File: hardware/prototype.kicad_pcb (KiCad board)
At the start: 2 copper layers, 200 x 200 mm, 111 parts, among them J1 CONN_02X20, SW1 SW_Push, SW10 SW_Push, SW11 SW_Push, SW12 SW_Push, SW13 SW_Push, SW14 SW_Push, SW15 SW_Push, SW16 SW_Push, SW17 SW_Push, SW18 SW_Push, SW19 SW_Push, SW2 SW_Push, SW20 SW_Push, SW21 SW_Push, SW22 SW_Push, SW23 SW_Push, SW24 SW_Push, SW25 SW_Push, SW26 SW_Push, SW3 SW_Push, SW4 SW_Push, SW5 SW_Push, SW6 SW_Push, SW7 SW_Push, SW8 SW_Push, SW9 SW_Push, U1 TLC5916, U10 SN74HC165N, U11 TLC5916, U2 TLC5916, U3 TLC5916, U4 SN74HC165N, U5 SN74HC165N, U6 TLC5916, U7 TLC5916, U8 TLC5916, U9 SN74HC165N

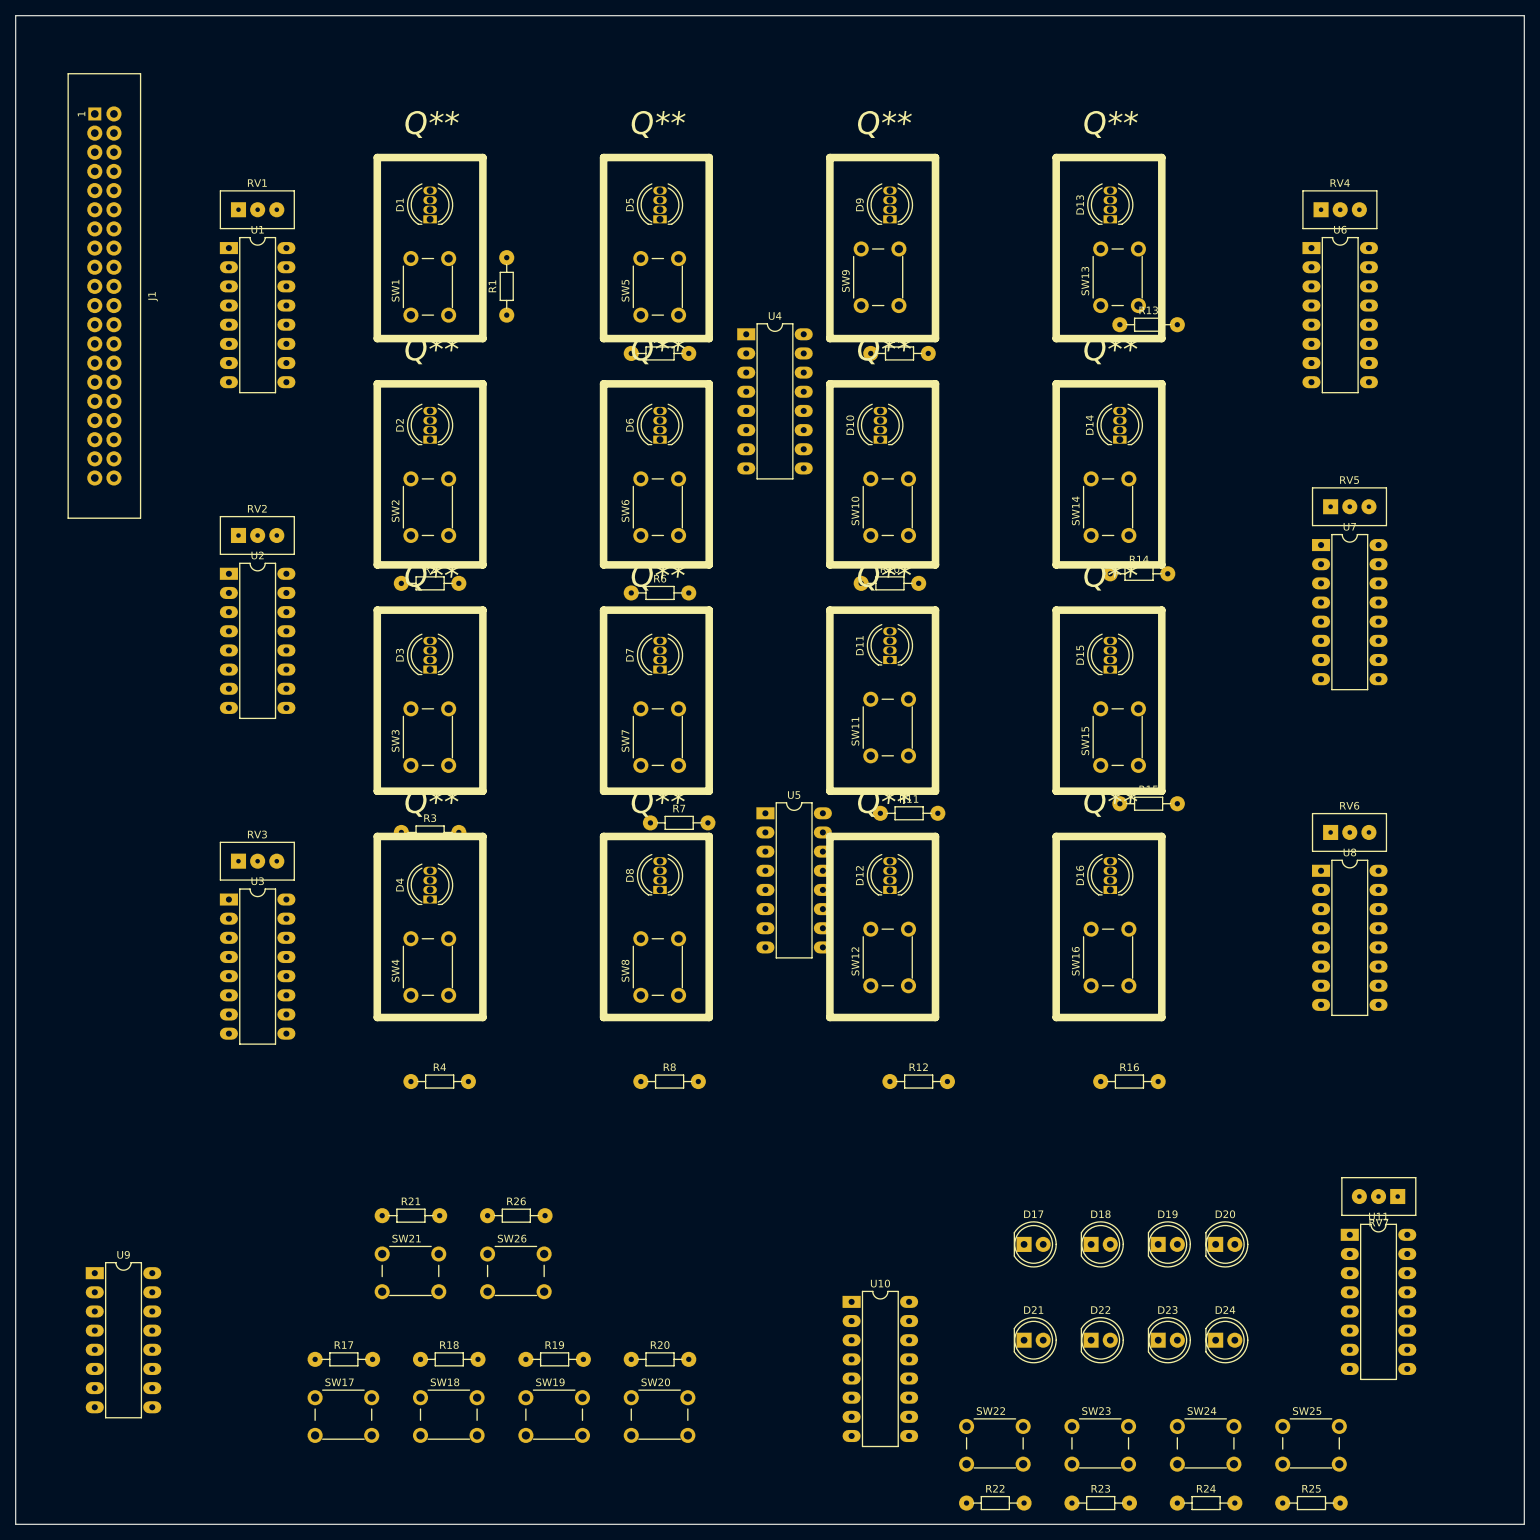
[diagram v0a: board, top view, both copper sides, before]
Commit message: More pcb stuff
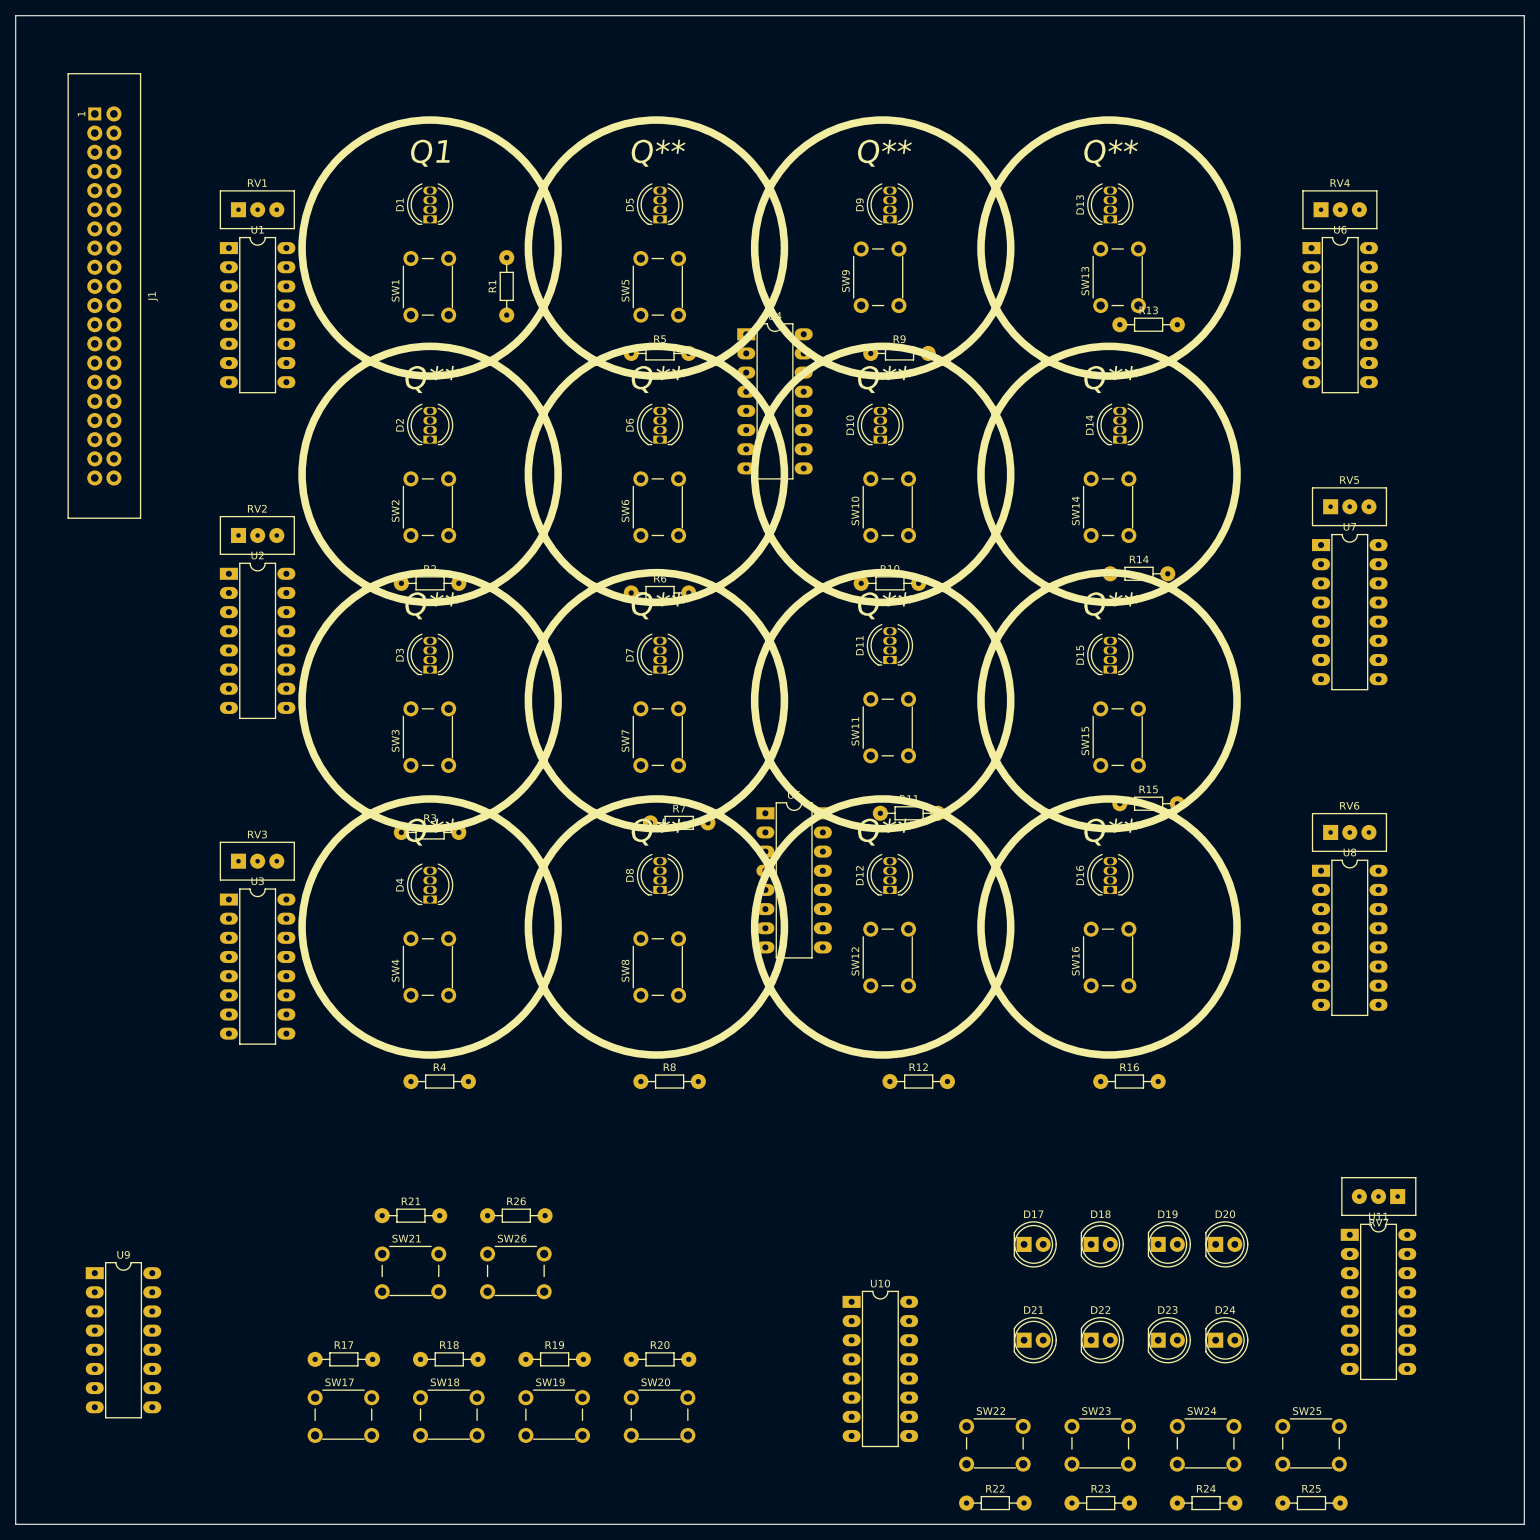
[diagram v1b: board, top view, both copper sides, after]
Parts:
- renumbered Q** to Q1
